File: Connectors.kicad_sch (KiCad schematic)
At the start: 17 parts, among them J1 A, J10 4900, J11 4900, J12 4900, J13 4900, J14 4900, J15 Conn_02x04_Odd_Even, J16 Conn_01x02, J17 Conn_01x02, J2 B, J3 C, J4 4900, J5 4900, J6 4900, J7 4900, J8 Temp, J9 4900

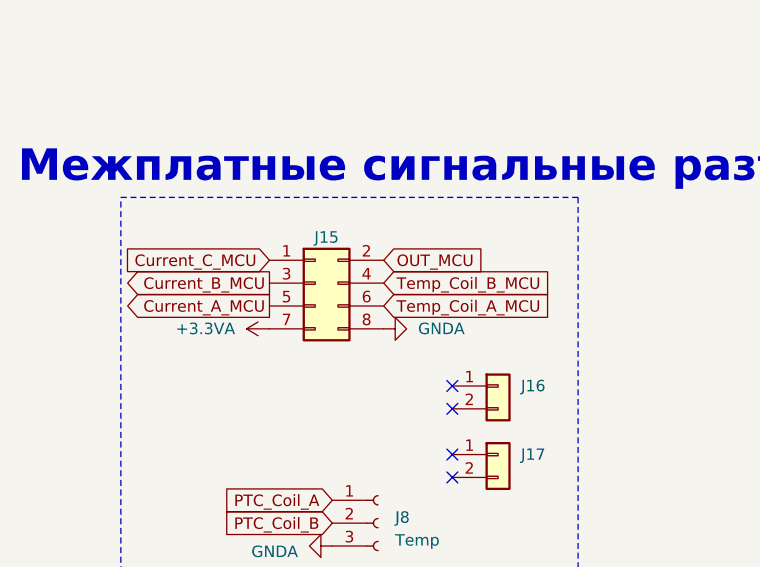
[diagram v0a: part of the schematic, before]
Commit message: Отправил на проверку в резонит
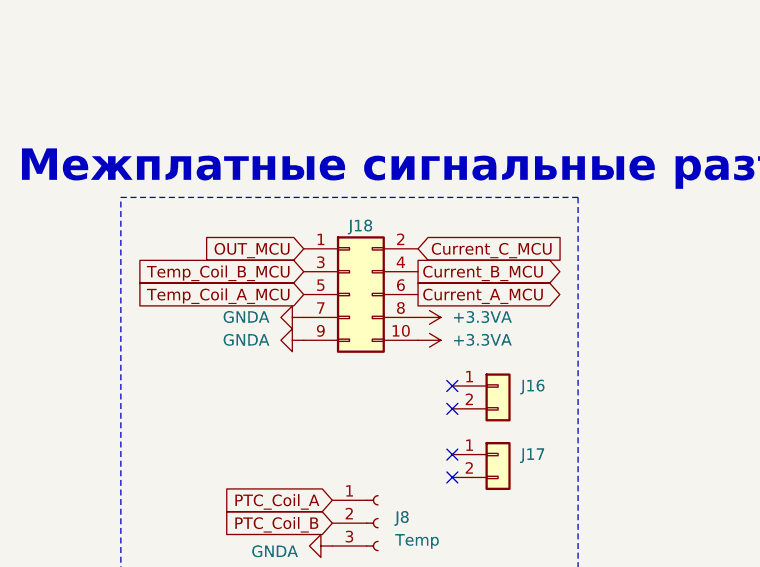
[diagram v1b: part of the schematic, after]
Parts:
- removed J15: Conn_02x04_Odd_Even, Connector_PinHeader_1.27mm:PinHeader_2x04_P1.27mm_Vertical, symbol Connector_Generic:Conn_02x04_Odd_Even
- added J18: Conn_02x05_Odd_Even, Connector_PinHeader_1.27mm:PinHeader_2x05_P1.27mm_Vertical, symbol Connector_Generic:Conn_02x05_Odd_Even
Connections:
- net +3.3VA: now also J18.10 (Pin_10), J18.8 (Pin_8)
- net Current_A_MCU: now also J18.6 (Pin_6)
- net Current_B_MCU: now also J18.4 (Pin_4)
- net Current_C_MCU: now also J18.2 (Pin_2)
- net GNDA: now also J18.7 (Pin_7), J18.9 (Pin_9)
- net OUT_MCU: now also J18.1 (Pin_1)
- net Temp_Coil_A_MCU: now also J18.5 (Pin_5)
- net Temp_Coil_B_MCU: now also J18.3 (Pin_3)

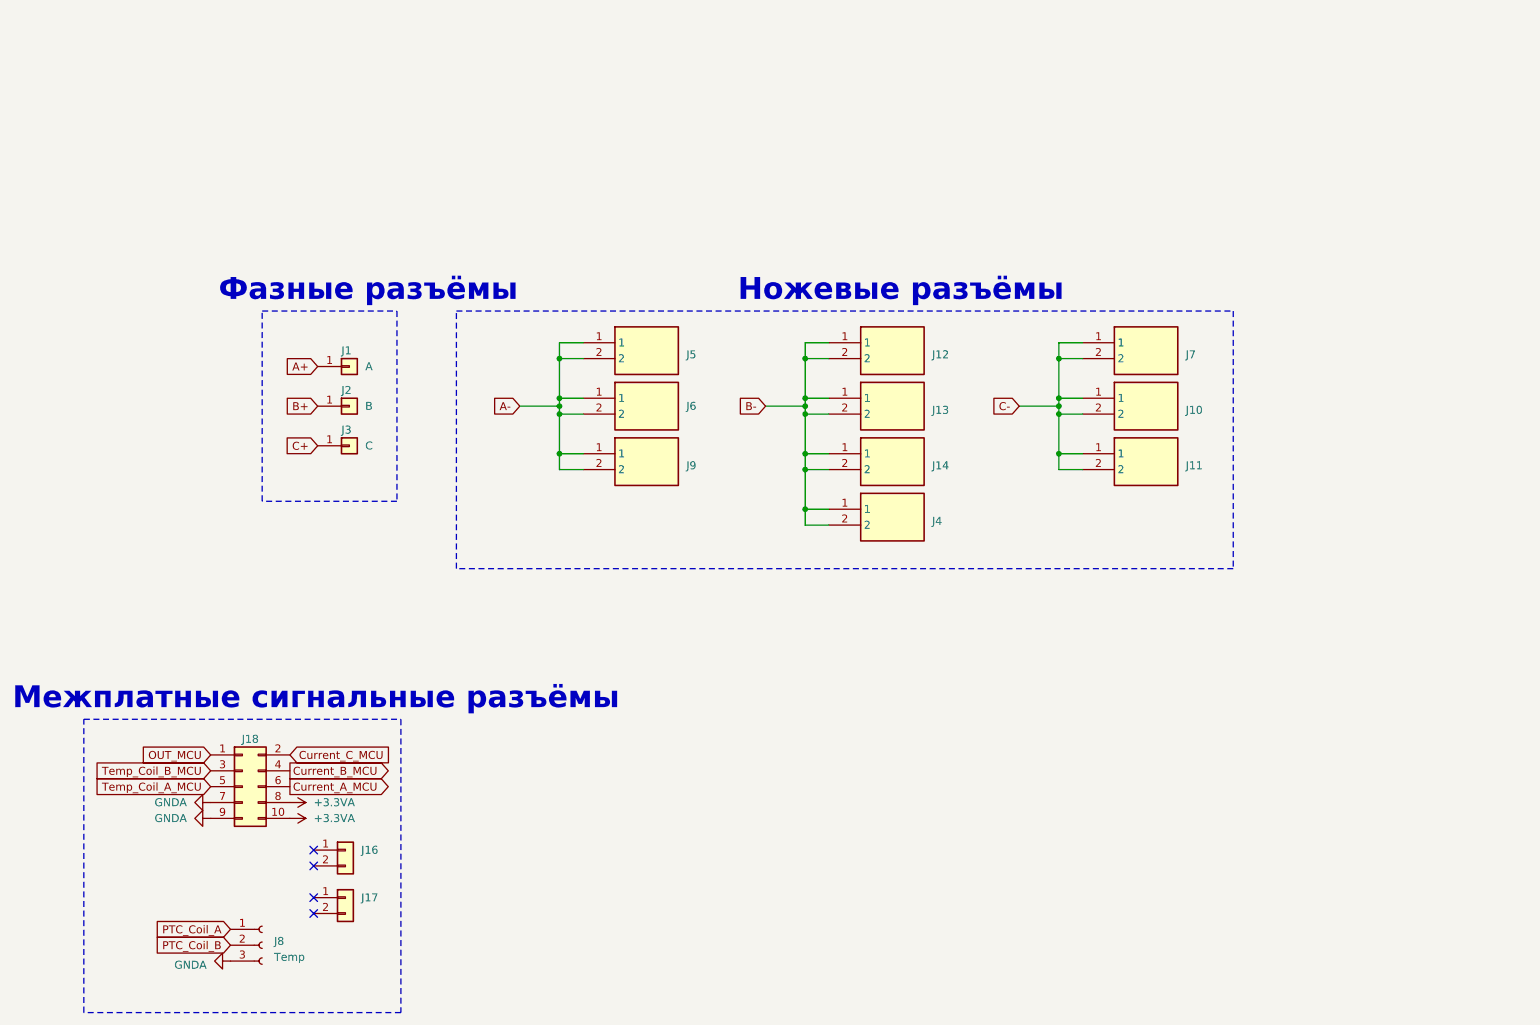
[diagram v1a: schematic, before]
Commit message: Изменения: добавил папку с отчетностью
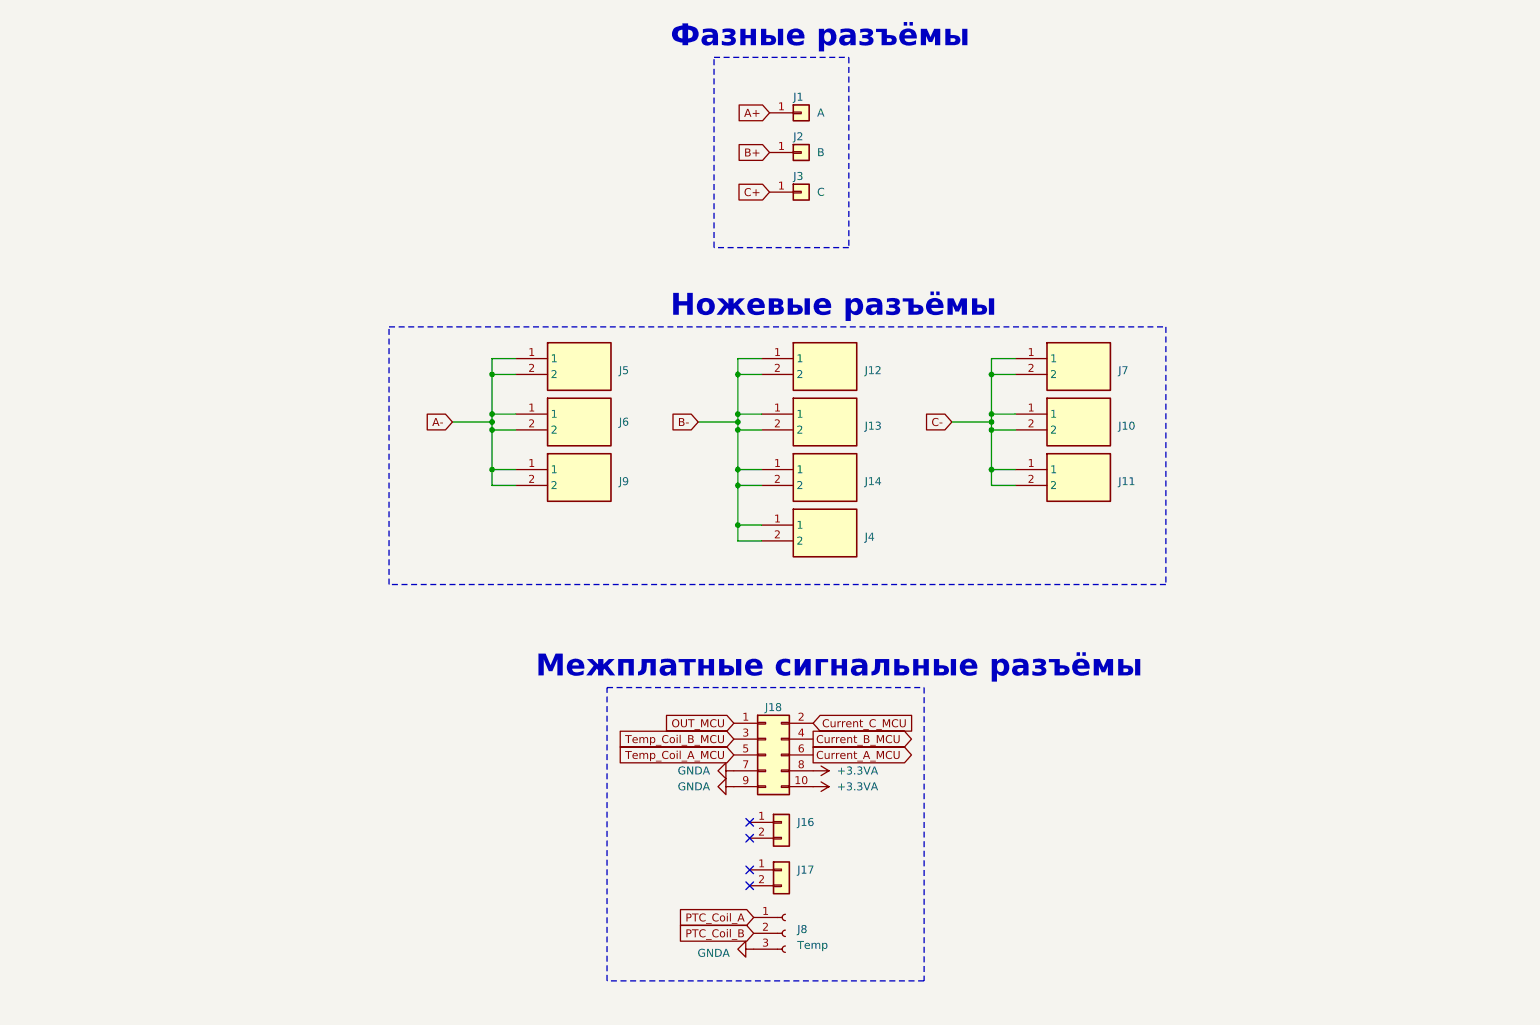
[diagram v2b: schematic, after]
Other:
- moved on the sheet: J1, J10, J11, J12, J13, J14, J16, J17, J18, J2, J3, J4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
